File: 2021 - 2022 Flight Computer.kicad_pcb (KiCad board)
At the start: 2 copper layers, 45 x 77 mm, 37 parts, among them IC1 TEENSY_4.0, IC2 XB24CZ7PIT-004, J1 Screw_Terminal_01x06, Q1 AOI21357, Q2 2N7002, Q3 2N7002, Q4 2N7002, Q5 AOI21357, U1 VXO7803-1000, U2 Flight-Computer_Adafruit_GPS_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, U3 ADXL345, U4 BMP280, U6 Memory_Flash_W25Q32JVSS

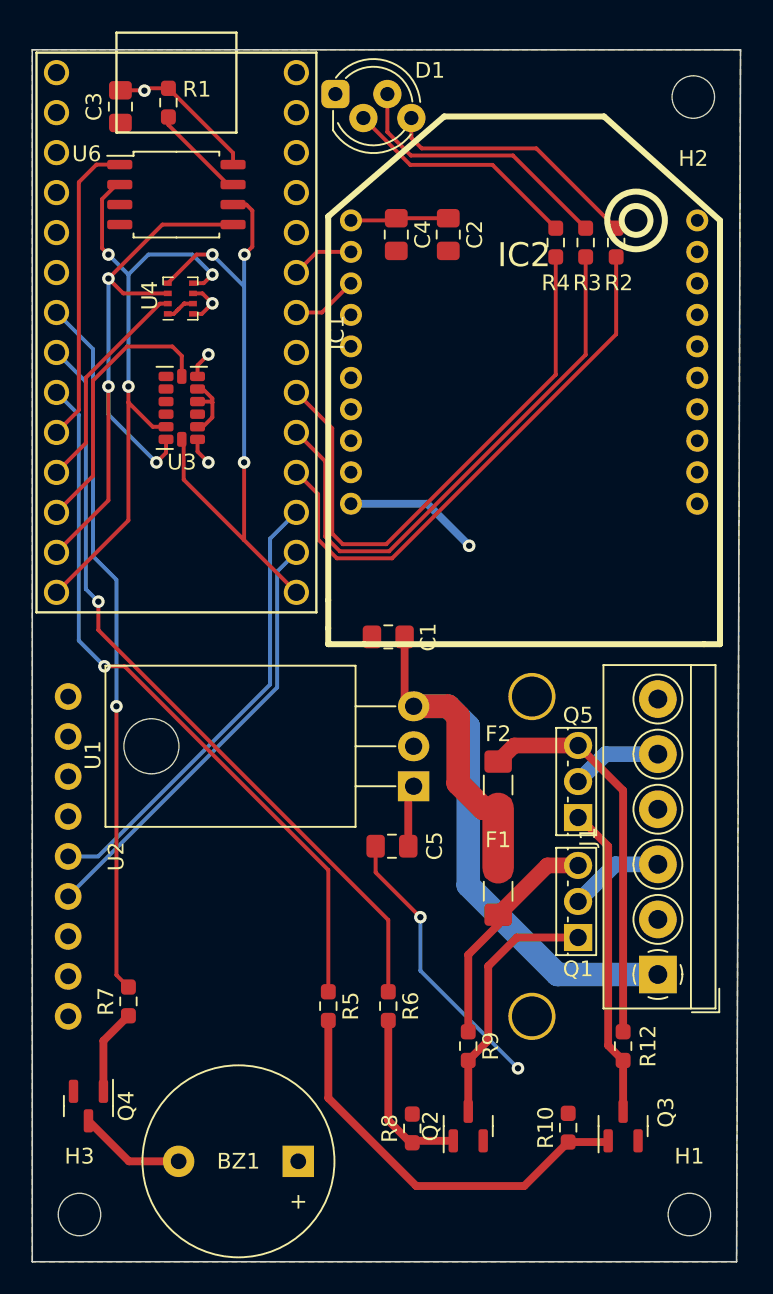
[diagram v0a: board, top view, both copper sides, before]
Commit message: New Gerbers
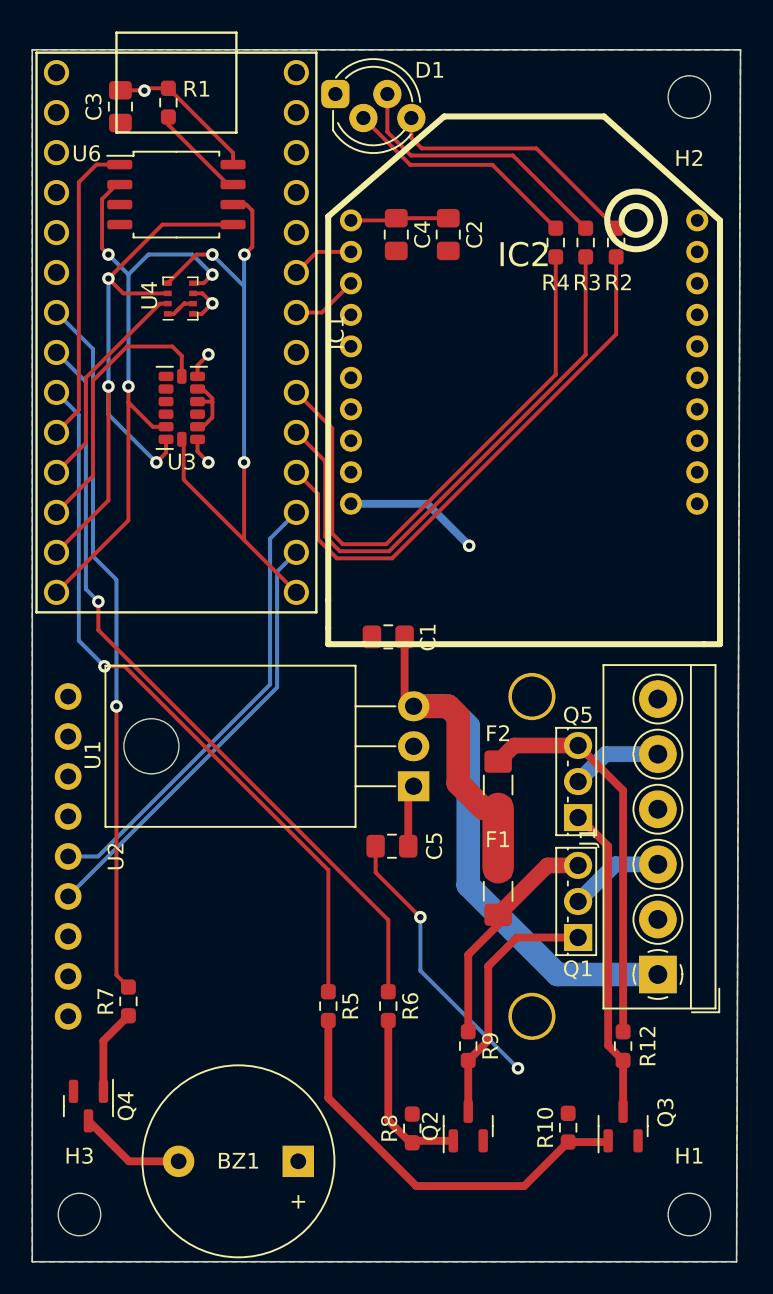
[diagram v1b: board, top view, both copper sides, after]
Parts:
- moved H2 0.25 mm to (113.8, 67.0)
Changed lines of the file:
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@@
     (pad_to_mask_clearance 0)
     (pcbplotparams
-      (layerselection 0x00010fc_ffffffff)
+      (layerselection 0x00010f0_ffffffff)
       (disableapertmacros false)
-      (usegerberextensions false)
+      (usegerberextensions true)
       (usegerberattributes true)
       (usegerberadvancedattributes true)
-      (creategerberjobfile true)
+      (creategerberjobfile false)
       (svguseinch false)
       (svgprecision 6)
@@
       (psa4output false)
       (plotreference true)
-      (plotvalue true)
+      (plotvalue false)
       (plotinvisibletext false)
       (sketchpadsonfab false)
@@
       (outputformat 1)
       (mirror false)
-      (drillshape 1)
+      (drillshape 0)
       (scaleselection 1)
-      (outputdirectory "")
+      (outputdirectory "New Gerbers/")
     )
   )
@@
     (fp_line (start 1 -0.625) (end 1 0.625) (layer "F.Fab") (width 0.1))
     (fp_line (start -1 0.625) (end -1 -0.625) (layer "F.Fab") (width 0.1))
-    (pad "1" smd roundrect locked (at -1.0375 0 180) (size 1.175 1.45) (layers "F.Cu" "F.Paste" "F.Mask") (roundrect_rratio 0.212766)
+    (pad "1" smd roundrect locked (at -1.0375 0 180) (size 1.175 1.45) (layers "F.Cu" "F.Paste" "F.Mask") (roundrect_rratio 0.2127659574)
       (net 60 "+BATT") (pintype "passive"))
-    (pad "2" smd roundrect locked (at 1.0375 0 180) (size 1.175 1.45) (layers "F.Cu" "F.Paste" "F.Mask") (roundrect_rratio 0.212766)
+    (pad "2" smd roundrect locked (at 1.0375 0 180) (size 1.175 1.45) (layers "F.Cu" "F.Paste" "F.Mask") (roundrect_rratio 0.2127659574)
       (net 4 "GND") (pintype "passive"))
     (model "${KICAD6_3DMODEL_DIR}/Capacitor_SMD.3dshapes/C_0805_2012Metric.wrl"
@@
     (fp_line (start -1 -0.625) (end 1 -0.625) (layer "F.Fab") (width 0.1))
     (fp_line (start 1 -0.625) (end 1 0.625) (layer "F.Fab") (width 0.1))
-    (pad "1" smd roundrect locked (at -1.0375 0 180) (size 1.175 1.45) (layers "F.Cu" "F.Paste" "F.Mask") (roundrect_rratio 0.212766)
+    (pad "1" smd roundrect locked (at -1.0375 0 180) (size 1.175 1.45) (layers "F.Cu" "F.Paste" "F.Mask") (roundrect_rratio 0.2127659574)
       (net 13 "+3V3") (pintype "passive"))
-    (pad "2" smd roundrect locked (at 1.0375 0 180) (size 1.175 1.45) (layers "F.Cu" "F.Paste" "F.Mask") (roundrect_rratio 0.212766)
+    (pad "2" smd roundrect locked (at 1.0375 0 180) (size 1.175 1.45) (layers "F.Cu" "F.Paste" "F.Mask") (roundrect_rratio 0.2127659574)
       (net 4 "GND") (pintype "passive"))
     (model "${KICAD6_3DMODEL_DIR}/Capacitor_SMD.3dshapes/C_0805_2012Metric.wrl"
@@
   )
   (footprint "MountingHole:MountingHole_2.7mm_M2.5" (layer "F.Cu")
-    (at 114 67)
+    (at 113.75 67)
     (descr "Mounting Hole 2.7mm, no annular, M2.5")
     (tags "mounting hole 2.7mm no annular m2.5")
@@
     (fp_line (start -1 -0.625) (end 1 -0.625) (layer "F.Fab") (width 0.1))
     (fp_line (start 1 0.625) (end -1 0.625) (layer "F.Fab") (width 0.1))
-    (pad "1" smd roundrect (at -1.0375 0 270) (size 1.175 1.45) (layers "F.Cu" "F.Paste" "F.Mask") (roundrect_rratio 0.212766)
+    (pad "1" smd roundrect (at -1.0375 0 270) (size 1.175 1.45) (layers "F.Cu" "F.Paste" "F.Mask") (roundrect_rratio 0.2127659574)
       (net 13 "+3V3") (pintype "passive"))
-    (pad "2" smd roundrect (at 1.0375 0 270) (size 1.175 1.45) (layers "F.Cu" "F.Paste" "F.Mask") (roundrect_rratio 0.212766)
+    (pad "2" smd roundrect (at 1.0375 0 270) (size 1.175 1.45) (layers "F.Cu" "F.Paste" "F.Mask") (roundrect_rratio 0.2127659574)
       (net 4 "GND") (pintype "passive"))
     (model "${KICAD6_3DMODEL_DIR}/Capacitor_SMD.3dshapes/C_0805_2012Metric.wrl"
@@
     (fp_line (start -1.6 0.8) (end -1.6 -0.8) (layer "F.Fab") (width 0.1))
     (fp_line (start -1.6 -0.8) (end 1.6 -0.8) (layer "F.Fab") (width 0.1))
-    (pad "1" smd roundrect locked (at -1.4875 0 270) (size 1.425 1.75) (layers "F.Cu" "F.Paste" "F.Mask") (roundrect_rratio 0.175439)
+    (pad "1" smd roundrect locked (at -1.4875 0 270) (size 1.425 1.75) (layers "F.Cu" "F.Paste" "F.Mask") (roundrect_rratio 0.1754392982)
       (net 60 "+BATT") (pintype "passive"))
-    (pad "2" smd roundrect locked (at 1.4875 0 270) (size 1.425 1.75) (layers "F.Cu" "F.Paste" "F.Mask") (roundrect_rratio 0.175439)
+    (pad "2" smd roundrect locked (at 1.4875 0 270) (size 1.425 1.75) (layers "F.Cu" "F.Paste" "F.Mask") (roundrect_rratio 0.1754392982)
       (net 26 "Net-(F1-Pad2)") (pintype "passive"))
     (model "${KICAD6_3DMODEL_DIR}/Fuse.3dshapes/Fuse_1206_3216Metric.wrl"
@@
     (fp_line (start -1 -0.625) (end 1 -0.625) (layer "F.Fab") (width 0.1))
     (fp_line (start 1 0.625) (end -1 0.625) (layer "F.Fab") (width 0.1))
-    (pad "1" smd roundrect (at -1.0375 0 270) (size 1.175 1.45) (layers "F.Cu" "F.Paste" "F.Mask") (roundrect_rratio 0.212766)
+    (pad "1" smd roundrect (at -1.0375 0 270) (size 1.175 1.45) (layers "F.Cu" "F.Paste" "F.Mask") (roundrect_rratio 0.2127659574)
       (net 13 "+3V3") (pintype "passive"))
-    (pad "2" smd roundrect (at 1.0375 0 270) (size 1.175 1.45) (layers "F.Cu" "F.Paste" "F.Mask") (roundrect_rratio 0.212766)
+    (pad "2" smd roundrect (at 1.0375 0 270) (size 1.175 1.45) (layers "F.Cu" "F.Paste" "F.Mask") (roundrect_rratio 0.2127659574)
       (net 4 "GND") (pintype "passive"))
     (model "${KICAD6_3DMODEL_DIR}/Capacitor_SMD.3dshapes/C_0805_2012Metric.wrl"
@@
     (fp_line (start 1 0.625) (end -1 0.625) (layer "F.Fab") (width 0.1))
     (fp_line (start -1 -0.625) (end 1 -0.625) (layer "F.Fab") (width 0.1))
-    (pad "1" smd roundrect locked (at -1.0375 0 90) (size 1.175 1.45) (layers "F.Cu" "F.Paste" "F.Mask") (roundrect_rratio 0.212766)
+    (pad "1" smd roundrect locked (at -1.0375 0 90) (size 1.175 1.45) (layers "F.Cu" "F.Paste" "F.Mask") (roundrect_rratio 0.2127659574)
       (net 4 "GND") (pintype "passive"))
-    (pad "2" smd roundrect locked (at 1.0375 0 90) (size 1.175 1.45) (layers "F.Cu" "F.Paste" "F.Mask") (roundrect_rratio 0.212766)
+    (pad "2" smd roundrect locked (at 1.0375 0 90) (size 1.175 1.45) (layers "F.Cu" "F.Paste" "F.Mask") (roundrect_rratio 0.2127659574)
       (net 13 "+3V3") (pintype "passive"))
     (model "${KICAD6_3DMODEL_DIR}/Capacitor_SMD.3dshapes/C_0805_2012Metric.wrl"
@@
     (fp_line (start -1.6 0.8) (end -1.6 -0.8) (layer "F.Fab") (width 0.1))
     (fp_line (start 1.6 0.8) (end -1.6 0.8) (layer "F.Fab") (width 0.1))
-    (pad "1" smd roundrect locked (at -1.4875 0 90) (size 1.425 1.75) (layers "F.Cu" "F.Paste" "F.Mask") (roundrect_rratio 0.175439)
+    (pad "1" smd roundrect locked (at -1.4875 0 90) (size 1.425 1.75) (layers "F.Cu" "F.Paste" "F.Mask") (roundrect_rratio 0.1754392982)
       (net 60 "+BATT") (pintype "passive"))
-    (pad "2" smd roundrect locked (at 1.4875 0 90) (size 1.425 1.75) (layers "F.Cu" "F.Paste" "F.Mask") (roundrect_rratio 0.175439)
+    (pad "2" smd roundrect locked (at 1.4875 0 90) (size 1.425 1.75) (layers "F.Cu" "F.Paste" "F.Mask") (roundrect_rratio 0.1754392982)
       (net 59 "Net-(F2-Pad2)") (pintype "passive"))
     (model "${KICAD6_3DMODEL_DIR}/Fuse.3dshapes/Fuse_1206_3216Metric.wrl"
